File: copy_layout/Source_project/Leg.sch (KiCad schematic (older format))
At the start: 10 parts, among them Q3 CSD19531KCS, Q4 CSD19531KCS, U4 IR2181, U5 LTS_15

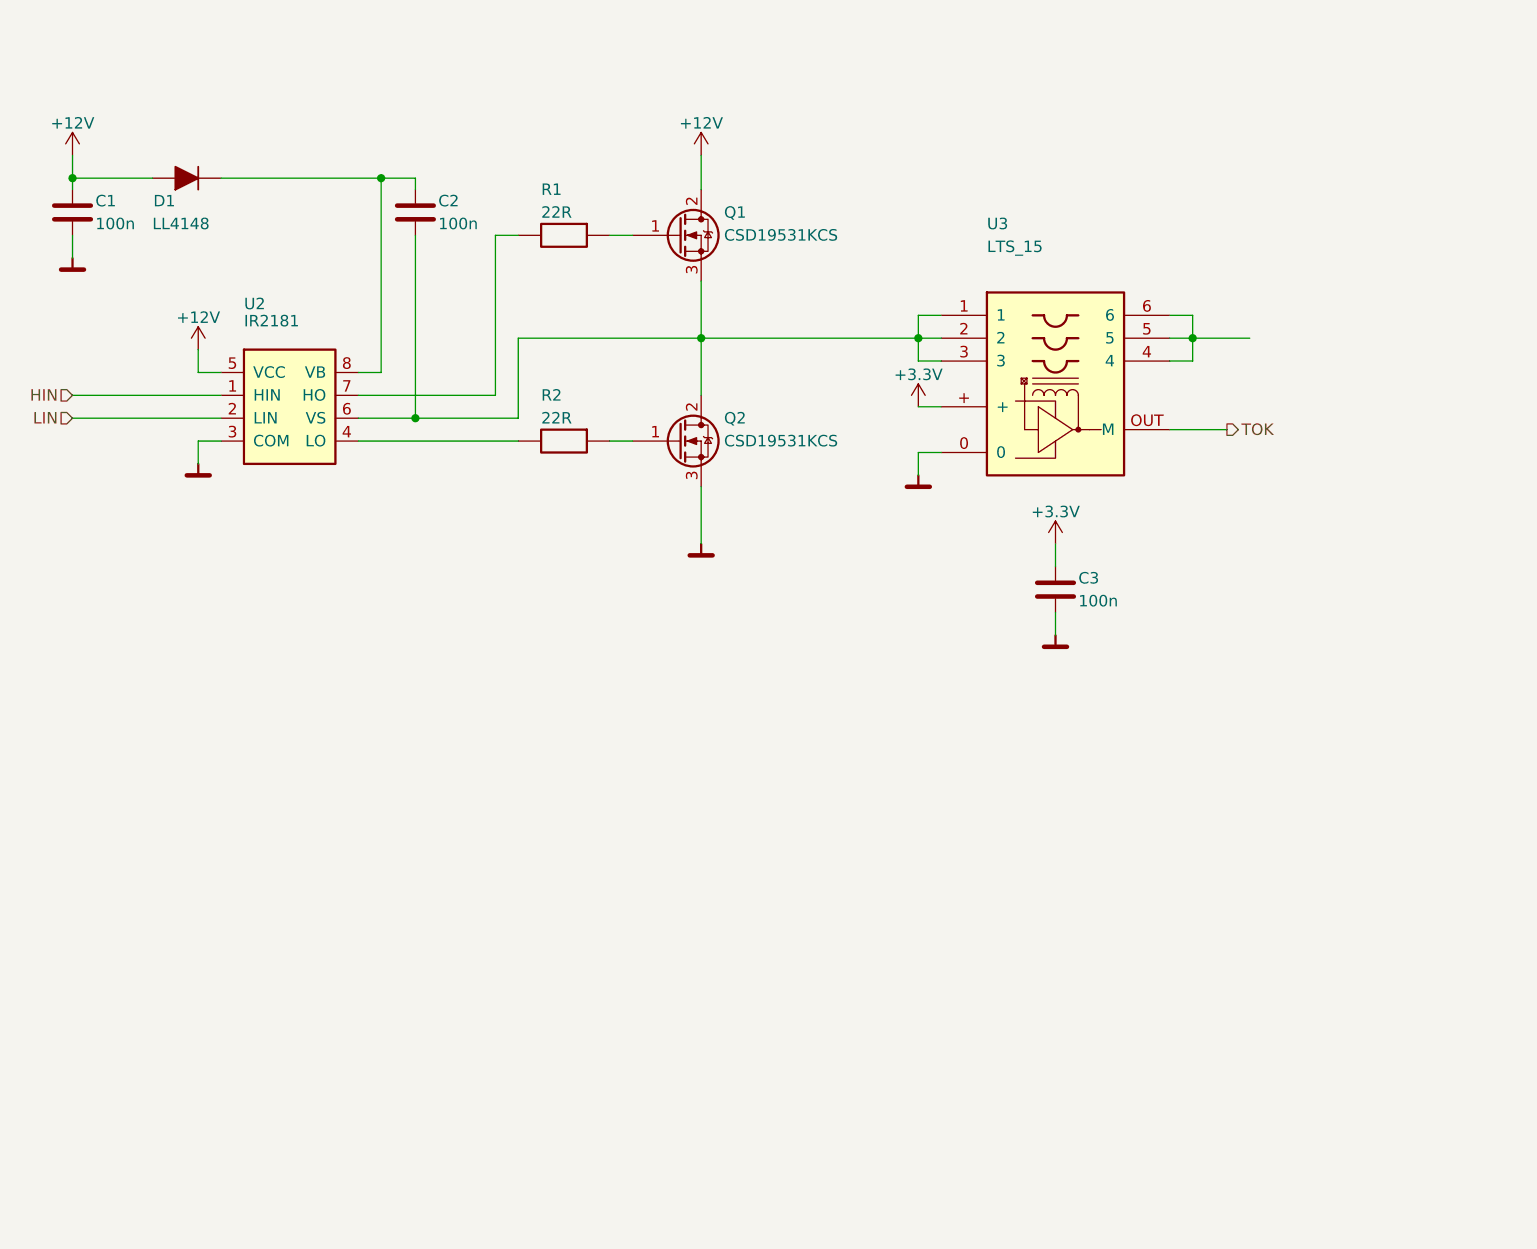
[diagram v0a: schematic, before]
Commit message: Modify test project
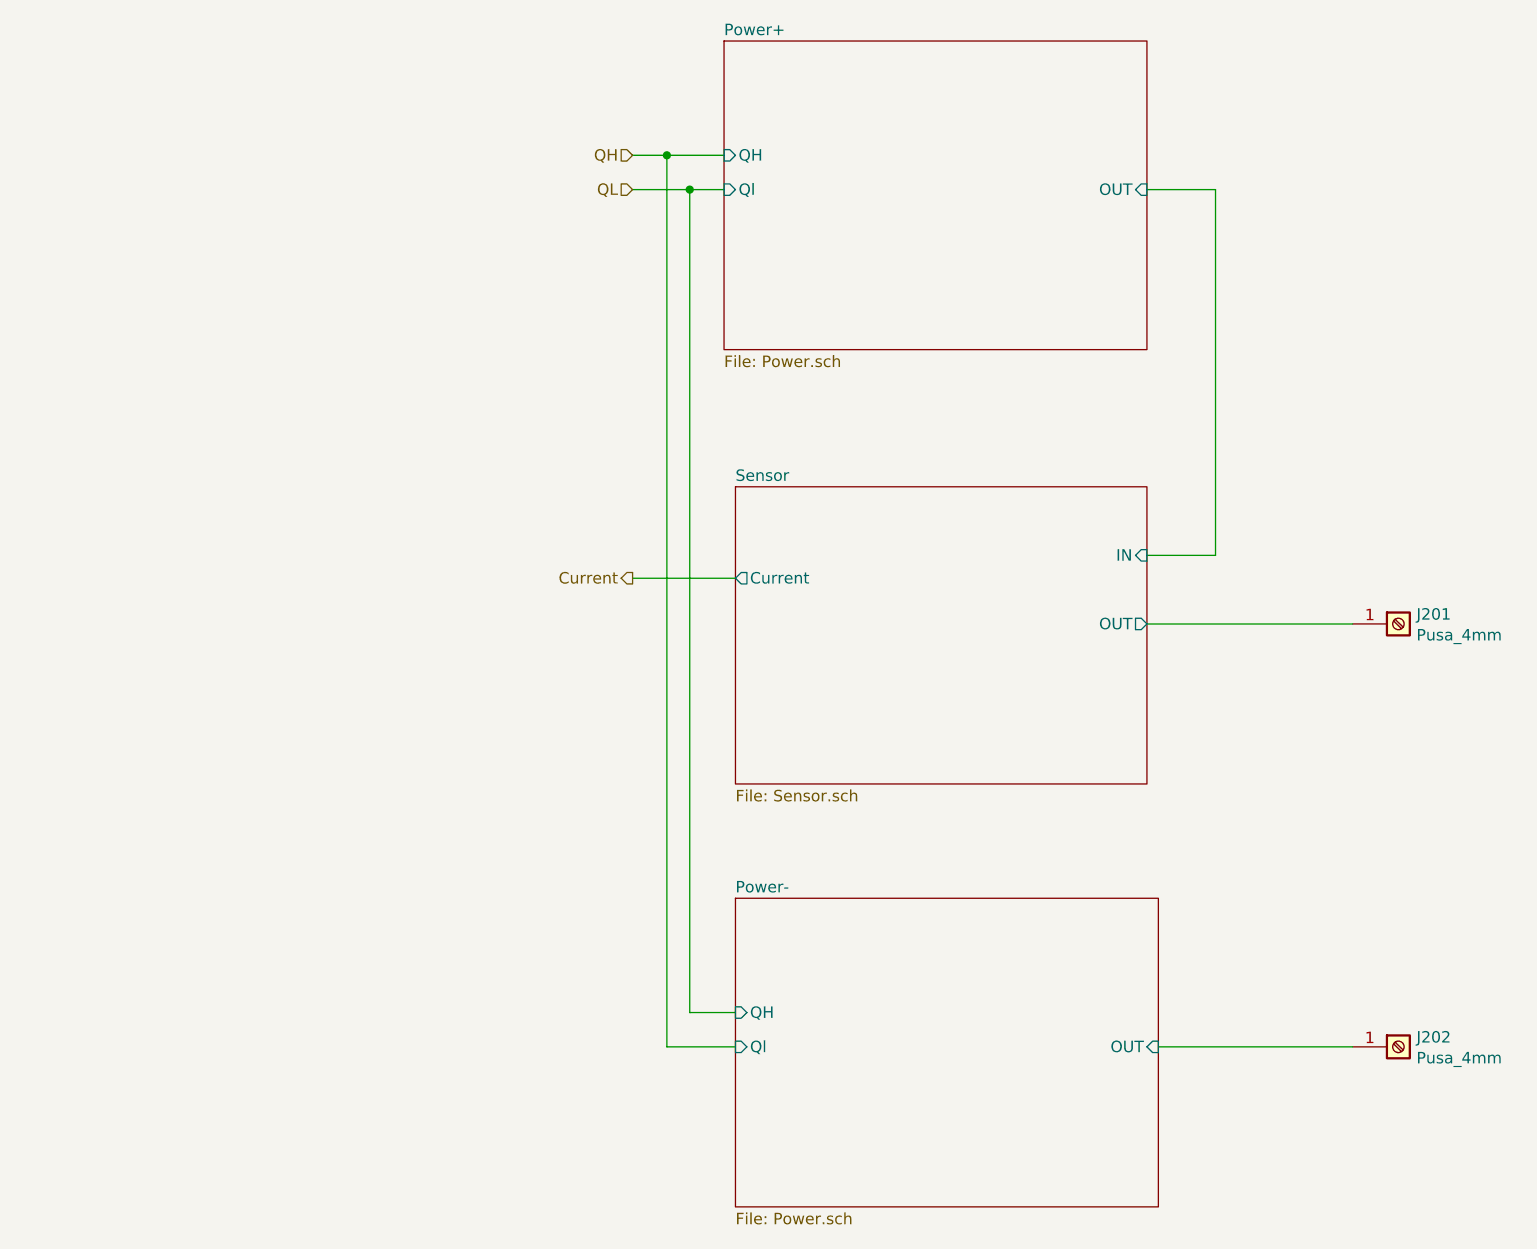
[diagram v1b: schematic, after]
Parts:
- removed C4, C5, C6: 100n, Passives:C1206M, symbol Passives:C1206
- removed D2: LL4148, Discretes:D_MiniMELF, symbol Discretes:LL4148
- removed Q3, Q4: CSD19531KCS, Discretes:TO-220, symbol Discretes:CSD19531KCS
- removed R3, R4: 22R, Passives:R1206M, symbol Passives:R1206
- removed U4: IR2181, Package_SO:SO8, symbol ICs:IR2181
- removed U5: LTS_15, Sensor_Current:LTS_15, symbol Sensor_Current:LTS_15
- added J201, J202: Pusa_4mm, Connector:Pusa_4mm, symbol Connector:Pusa_4mm
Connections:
- new net Power-/OUT: J202.1 (Pin_1)
- new net Sensor/OUT: J201.1 (Pin_1)
